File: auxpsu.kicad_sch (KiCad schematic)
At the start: 39 parts, among them J4 1mm, U2 TOP264VG, U3 FODM217D, U4 TL431DBZ

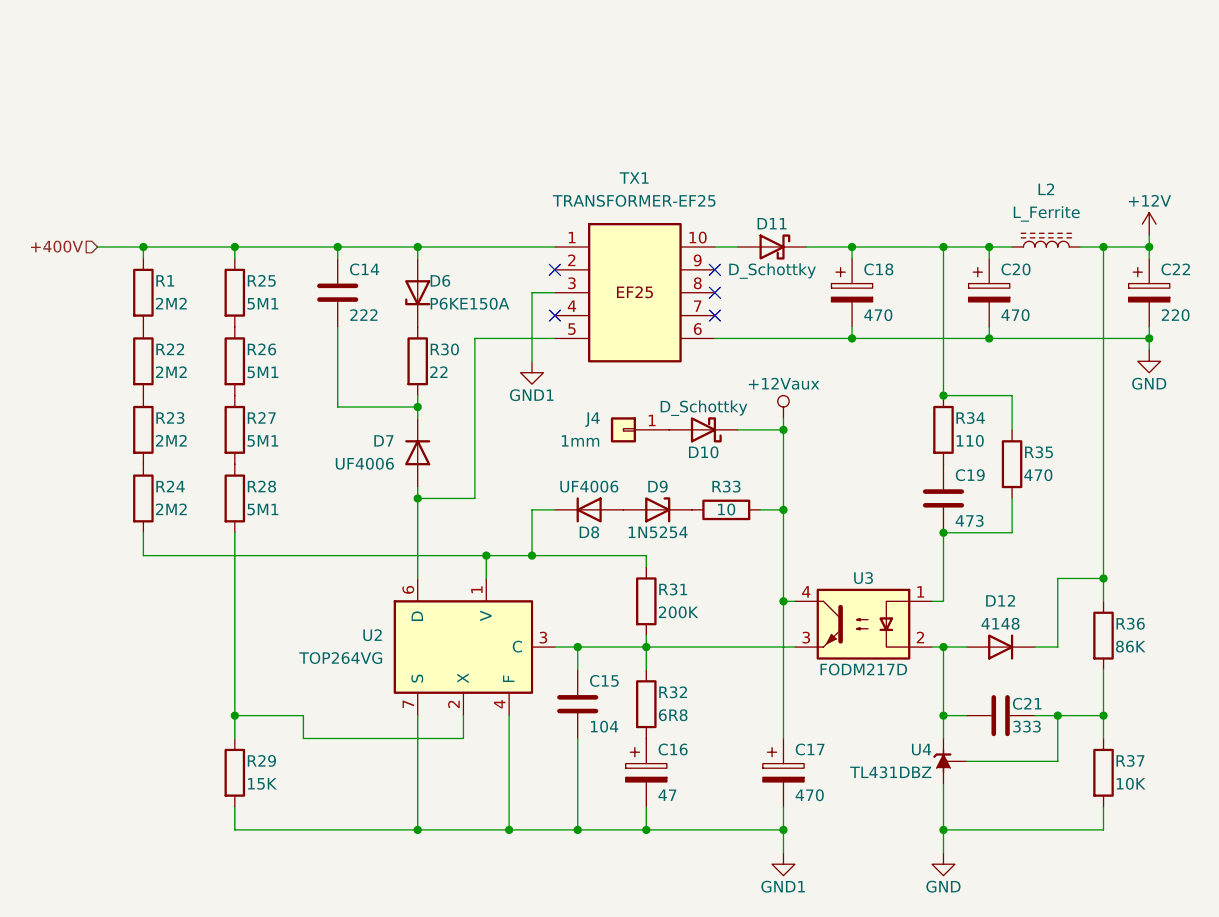
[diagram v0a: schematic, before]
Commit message: Schematic & PCB updated.
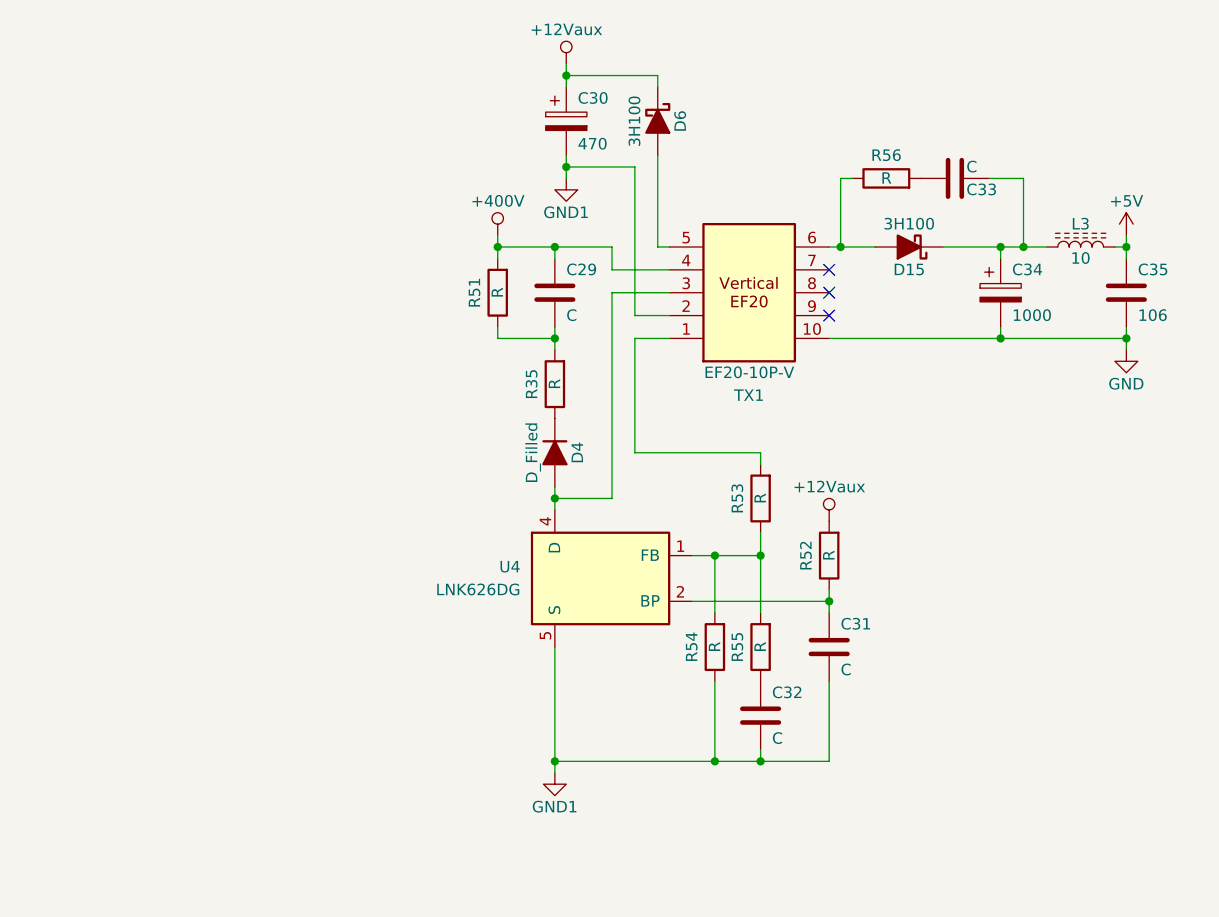
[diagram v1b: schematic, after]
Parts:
- removed C14: 222, Capacitor_THT:C_Disc_D12.5mm_W5.0mm_P7.50mm, symbol Device:C
- removed C15: 104, Capacitor_SMD:C_0805_2012Metric, symbol Device:C
- removed C16: 47, Capacitor_THT:CP_Radial_D5.0mm_P2.00mm, symbol Device:C_Polarized
- removed C17, C18, C20: 470, Capacitor_THT:CP_Radial_D10.0mm_P5.00mm, symbol Device:C_Polarized
- removed C19: 473, Capacitor_SMD:C_0805_2012Metric, symbol Device:C
- removed C21: 333, Capacitor_SMD:C_0805_2012Metric, symbol Device:C
- removed C22: 220, Capacitor_THT:CP_Radial_D10.0mm_P5.00mm, symbol Device:C_Polarized
- removed D10, D11: D_Schottky, Diode_THT:D_DO-201AD_P5.08mm_Vertical_KathodeUp, symbol Device:D_Schottky
- removed D12: 4148, Diode_SMD:D_SOD-123, symbol Device:D
- removed D6: P6KE150A, Diode_THT:D_DO-15_P5.08mm_Vertical_KathodeUp, symbol Device:D_Zener
- removed D7: UF4006, Diode_THT:D_DO-41_SOD81_P5.08mm_Vertical_KathodeUp, symbol Device:D
- removed D8: UF4006, Diode_SMD:D_SOD-123, symbol Device:D
- removed D9: 1N5254, Diode_SMD:D_SOD-123, symbol Device:D_Zener
- removed J4: 1mm, Connector_Pin:Pin_D1.0mm_L10.0mm_LooseFit, symbol Connector_Generic:Conn_01x01
- removed L2: L_Ferrite, HR Parts:INDUCTOR_SMD_7x7, symbol Device:L_Ferrite
- removed R1, R22, R23, R24: 2M2, Resistor_SMD:R_0805_2012Metric, symbol Device:R
- removed R25, R26, R27, R28: 5M1, Resistor_SMD:R_0805_2012Metric, symbol Device:R
- removed R29: 15K, Resistor_SMD:R_0805_2012Metric, symbol Device:R
- removed R30: 22, Resistor_THT:R_Axial_DIN0414_L11.9mm_D4.5mm_P5.08mm_Vertical, symbol Device:R
- removed R31: 200K, Resistor_SMD:R_0805_2012Metric, symbol Device:R
- removed R32: 6R8, Resistor_SMD:R_0805_2012Metric, symbol Device:R
- removed R33: 10, Resistor_SMD:R_0805_2012Metric, symbol Device:R
- removed R34: 110, Resistor_SMD:R_0805_2012Metric, symbol Device:R
- removed R36: 86K, Resistor_SMD:R_0805_2012Metric, symbol Device:R
- removed R37: 10K, Resistor_SMD:R_0805_2012Metric, symbol Device:R
- removed TX1: TRANSFORMER-EF25, HR Parts:TRANSFORMER_EF25_HORIZONTAL, symbol HR-parts:TRANSFORMER-EF25
- removed U2: TOP264VG, Package_DIP:PowerIntegrations_eDIP-12B, symbol Regulator_Switching:TOP264VG
- removed U3: FODM217D, Package_DIP:DIP-4_W10.16mm, symbol Isolator:FODM217D
- removed U4: TL431DBZ, Package_TO_SOT_SMD:SOT-23, symbol Reference_Voltage:TL431DBZ
- added C29: C, Capacitor_SMD:C_1206_3216Metric, symbol Device:C
- added C30: 470, Capacitor_THT:CP_Radial_D10.0mm_P5.00mm, symbol Device:C_Polarized
- added C31, C32, C33: C, Capacitor_SMD:C_0805_2012Metric, symbol Device:C
- added C34: 1000, Capacitor_THT:CP_Radial_D10.0mm_P5.00mm, symbol Device:C_Polarized
- added C35: 106, Capacitor_SMD:C_1210_3225Metric, symbol Device:C
- added D15, D6: 3H100, Diode_SMD:D_SMB, symbol Device:D_Schottky_Filled
- added D4: D_Filled, Diode_SMD:D_SOD-123, symbol Device:D_Filled
- added L3: 10, HR_Parts:INDUCTOR_SMD_4x4, symbol Device:L_Ferrite
- added R51: R, Resistor_SMD:R_1206_3216Metric, symbol Device:R
- added R52, R53, R54, R55, R56: R, Resistor_SMD:R_0805_2012Metric, symbol Device:R
- added TX1: EF20-10P-V, HR_Parts:TRANSFORMER-EF20-10P-V, symbol HR Parts:TRANSFORMER-EF20-10P-V
- added U4: LNK626DG, Package_SO:PowerIntegrations_SO-8C, symbol Regulator_Switching:LNK626DG
- R35: value 470 -> R
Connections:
- net +12Vaux: now also C30.1, D6.1 (K), R52.2
- net +400V: now also C29.1, R51.2, TX1.4
- net GND: now also C34.2, C35.2, TX1.10
- net GND1: now also C30.2, C31.2, C32.2, R54.1, TX1.2, U4.5 (S), U4.6 (S), U4.7 (S), U4.8 (S)
- net at R35.1: now also D4.1 (K)
- net at R35.2: now also C29.2, R51.1
- new net: D4.2 (A), TX1.3, U4.4 (D)
- new net: D15.2 (A), R56.1, TX1.6
- new net: C33.1, R56.2
- new net: R53.2, TX1.1
- new net: D6.2 (A), TX1.5
- new net: C32.1, R55.1
- new net: R53.1, R54.2, R55.2, U4.1 (FB)
- new net: C31.1, R52.1, U4.2 (BP)
- new net: C33.2, C34.1, D15.1 (K), L3.1
- new net +5V: C35.1, L3.2
- no-connect marks 5 -> 3
